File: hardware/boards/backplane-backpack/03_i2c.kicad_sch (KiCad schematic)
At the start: 33 parts, among them J3 I2C CH0 (TBD), J4 I2C CH1 (TBD), J5 I2C CH2 (TBD), J6 I2C CH3 (TBD), J7 I2C CH4 (TBD), J8 I2C CH5 (TBD), U2 TCA9548APWR

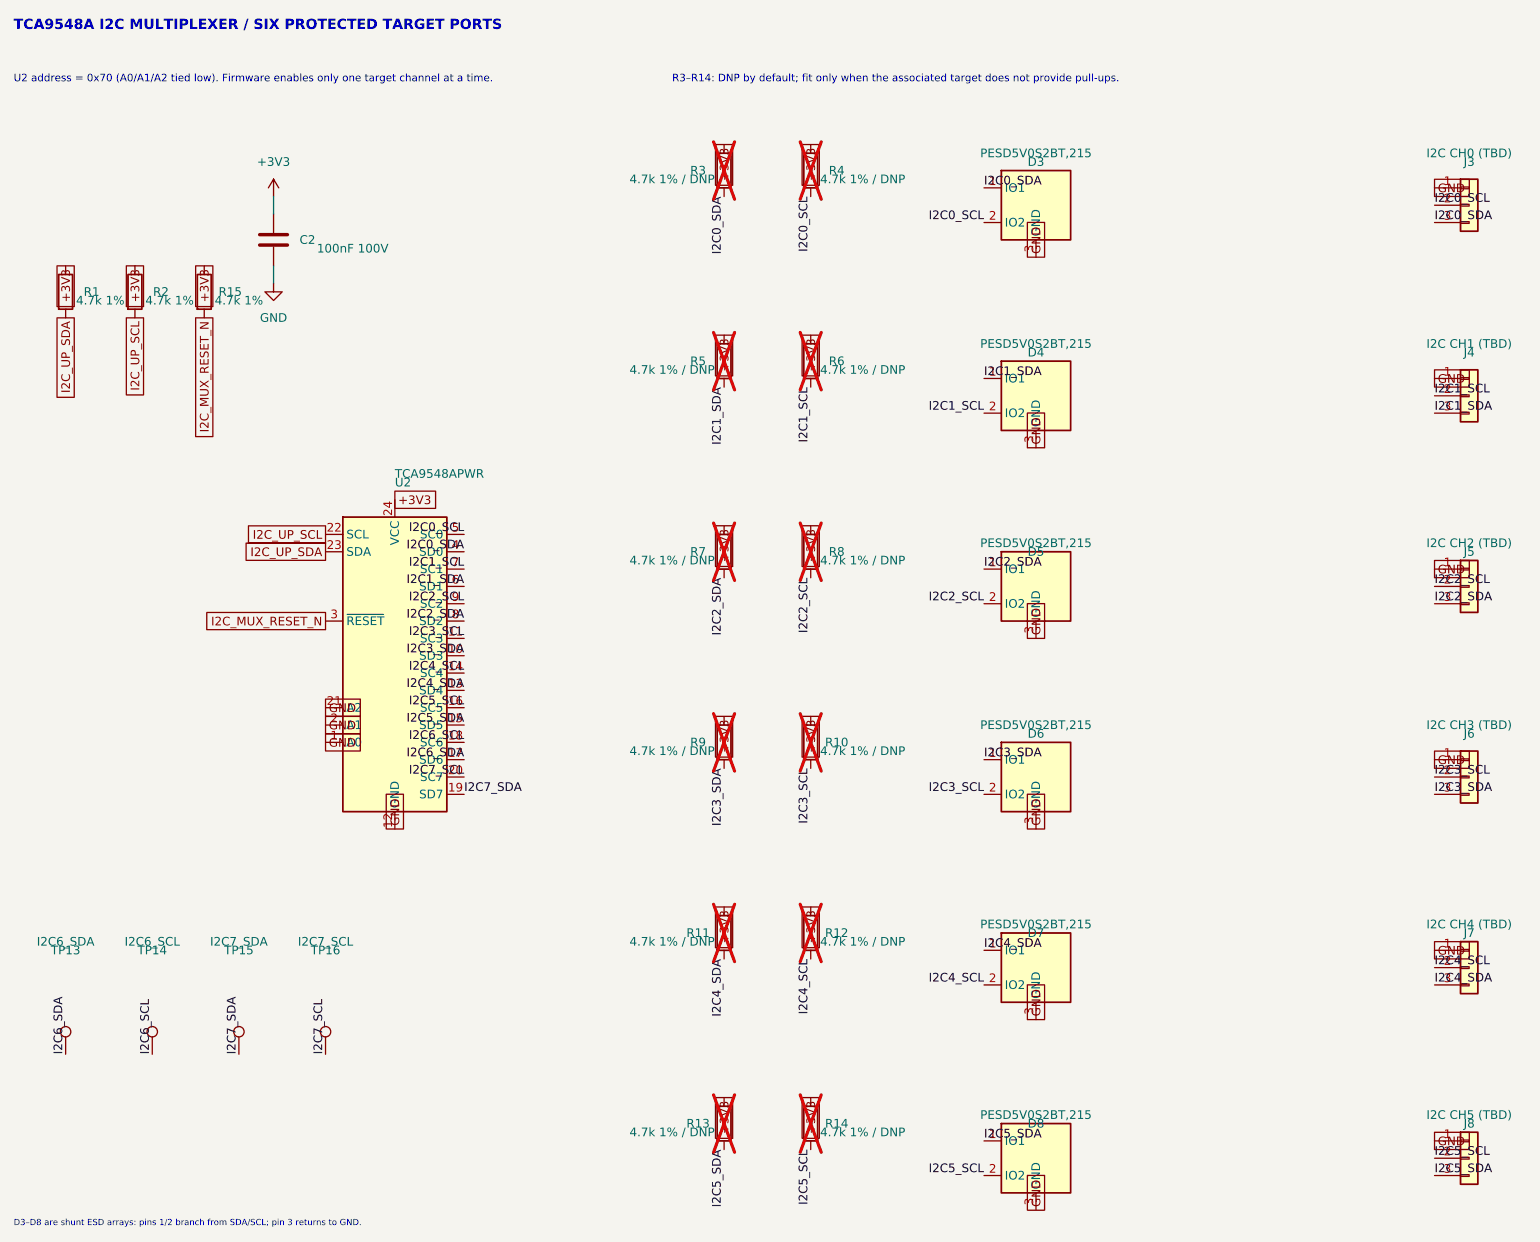
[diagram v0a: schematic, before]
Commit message: chore: checkpoint workspace changes
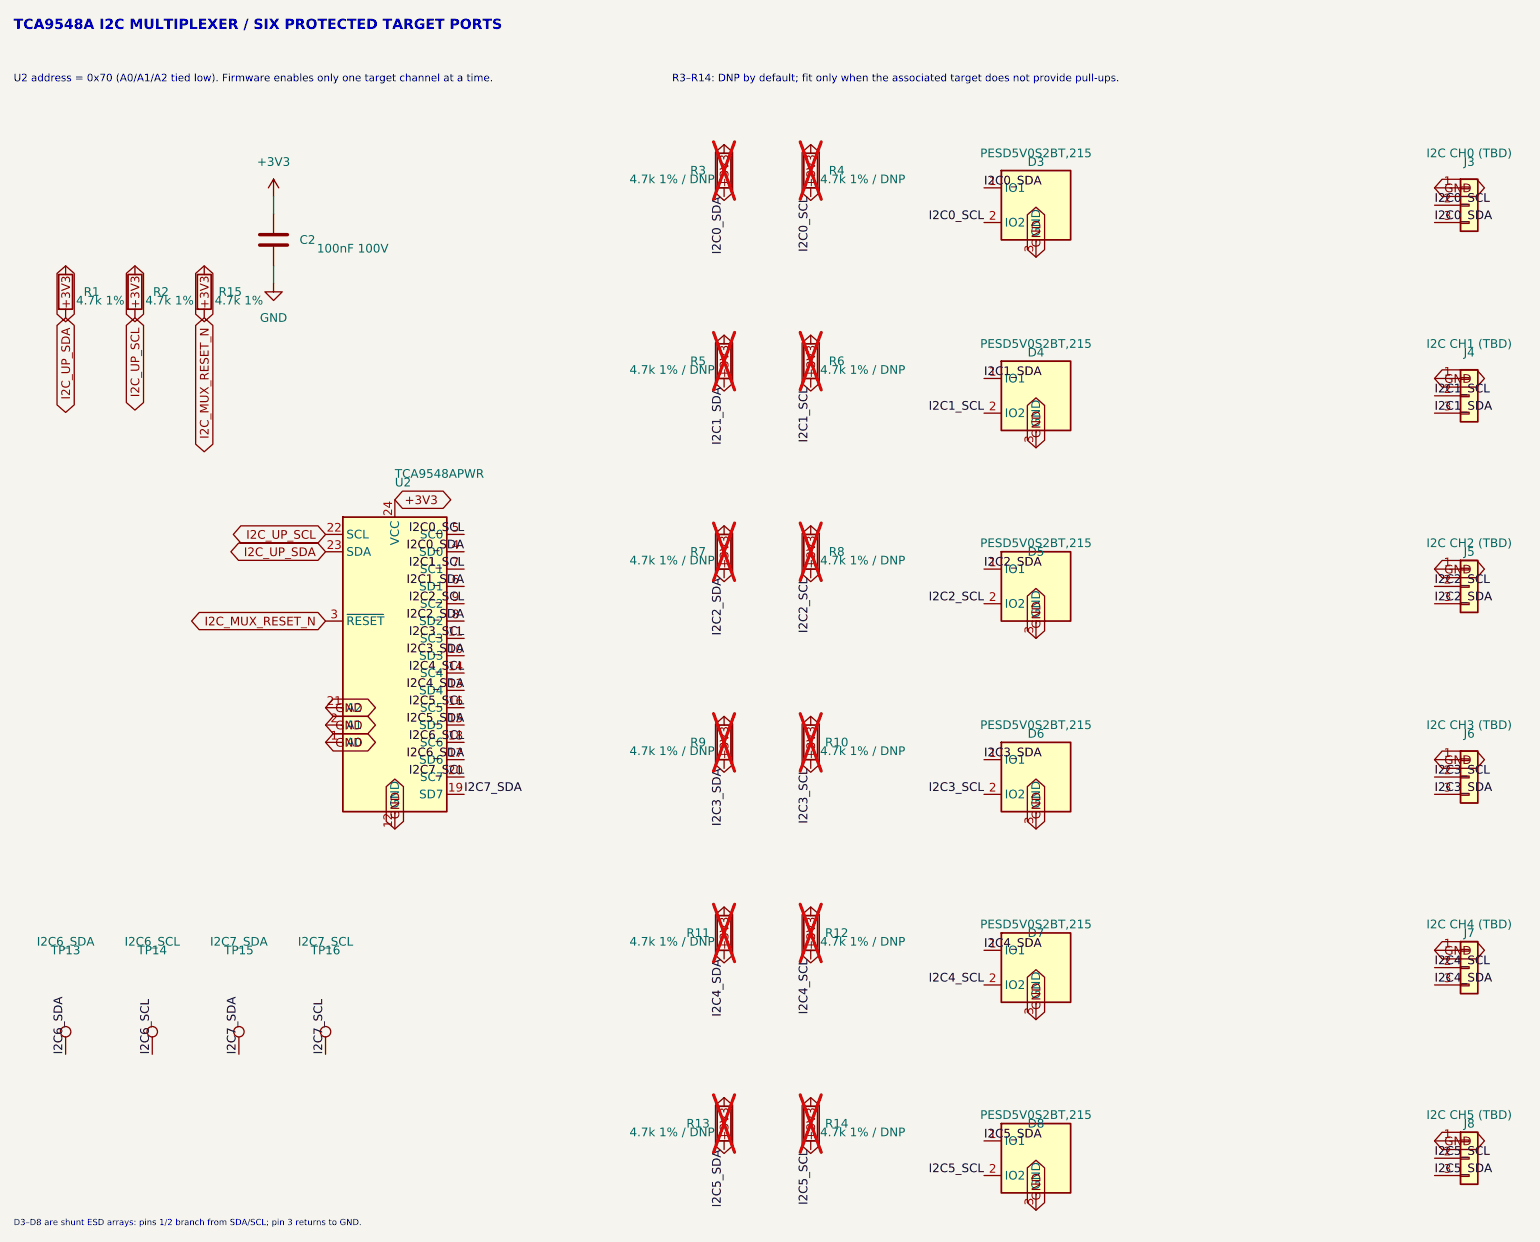
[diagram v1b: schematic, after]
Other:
- company: (none) -> Karl Quinsland
- title: I2C Multiplexer and Ports -> Backplane Backpack
